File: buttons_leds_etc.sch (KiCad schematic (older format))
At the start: 10 parts, among them SW2 SW_Push, SW3 SW_Push

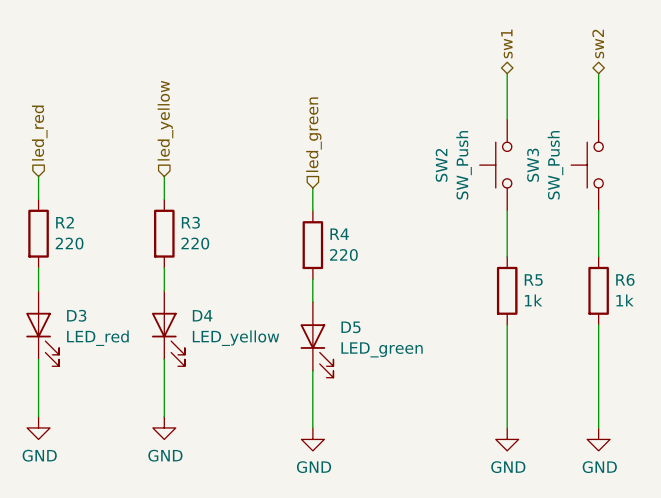
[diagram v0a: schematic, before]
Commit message: update front endu do termopary i przełącznika zasilającego
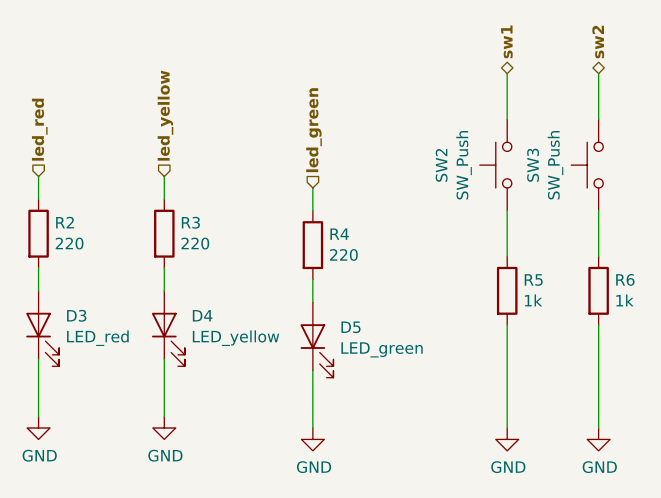
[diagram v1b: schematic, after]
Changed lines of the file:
@@
 Wire Wire Line
 	3450 2950 3450 2850
-Text HLabel 2250 2400 1    50   Input ~ 0
+Text HLabel 2250 2400 1    50   Input ~ 6
 led_red
 Wire Wire Line
 	2250 2500 2250 2400
-Text HLabel 2800 2400 1    50   Input ~ 0
+Text HLabel 2800 2400 1    50   Input ~ 6
 led_yellow
 Wire Wire Line
 	2800 2400 2800 2500
-Text HLabel 3450 2450 1    50   Input ~ 0
+Text HLabel 3450 2450 1    50   Input ~ 6
 led_green
 Wire Wire Line
@@
 Wire Wire Line
 	4700 3500 4700 3050
-Text HLabel 4300 1950 1    50   BiDi ~ 0
+Text HLabel 4300 1950 1    50   BiDi ~ 6
 sw1
 Wire Wire Line
 	4300 2150 4300 1950
-Text HLabel 4700 1950 1    50   BiDi ~ 0
+Text HLabel 4700 1950 1    50   BiDi ~ 6
 sw2
 Wire Wire Line
